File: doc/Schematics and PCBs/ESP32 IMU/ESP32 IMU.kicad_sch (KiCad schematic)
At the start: 7 parts, among them J1 +5V, U1 BA50JC5T

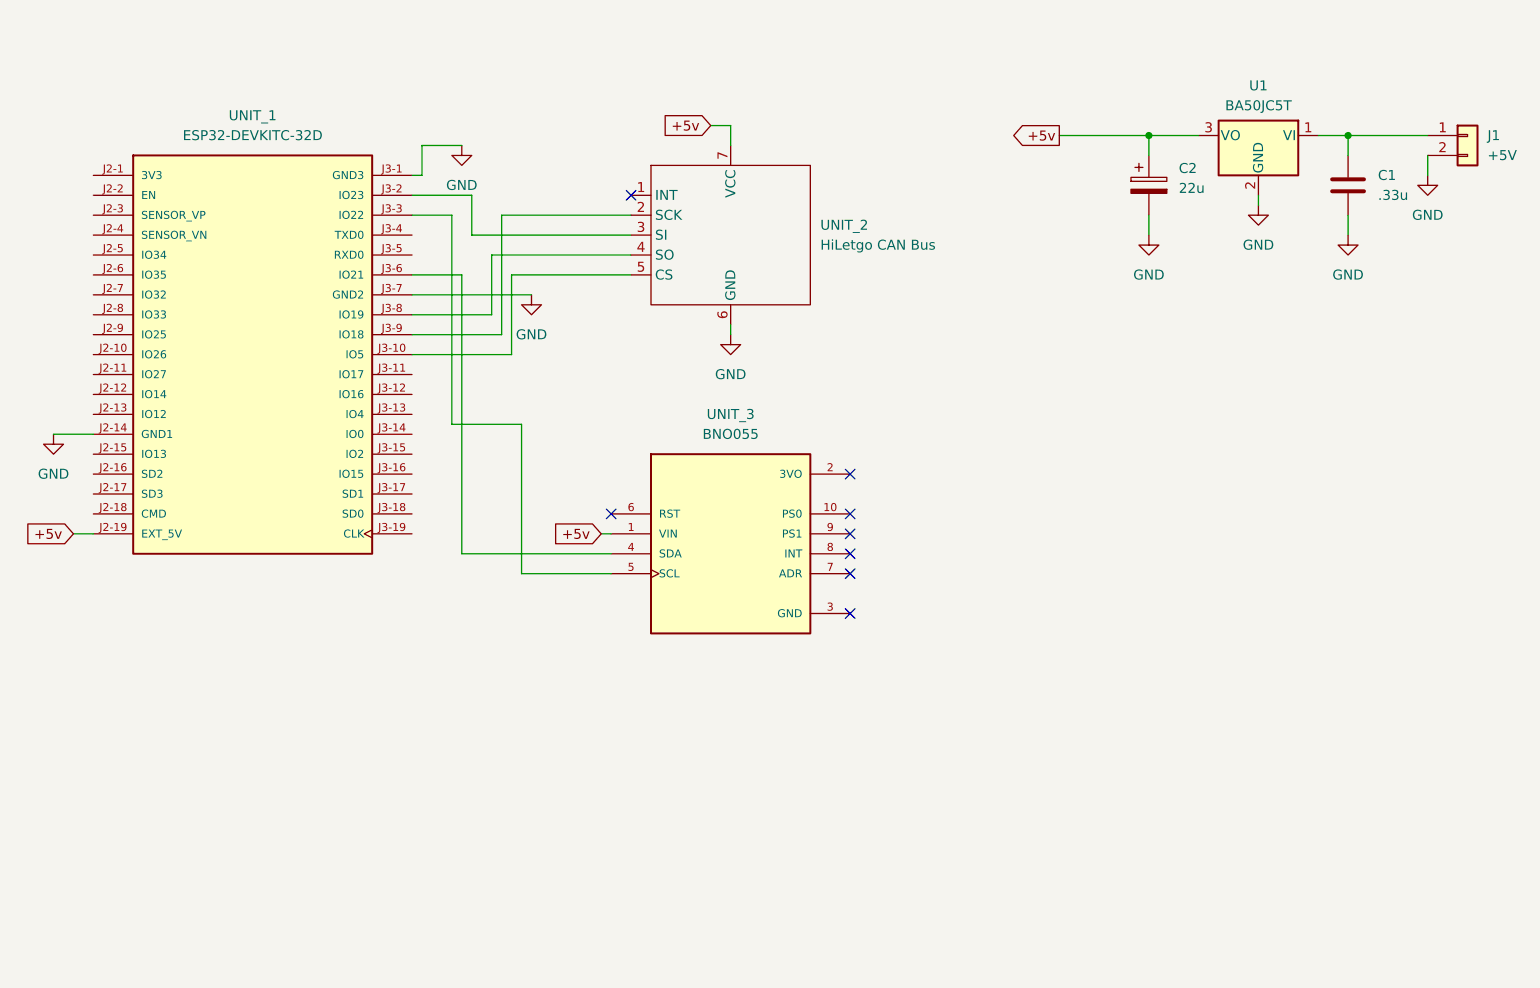
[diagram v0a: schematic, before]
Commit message: Final Touches on IMU
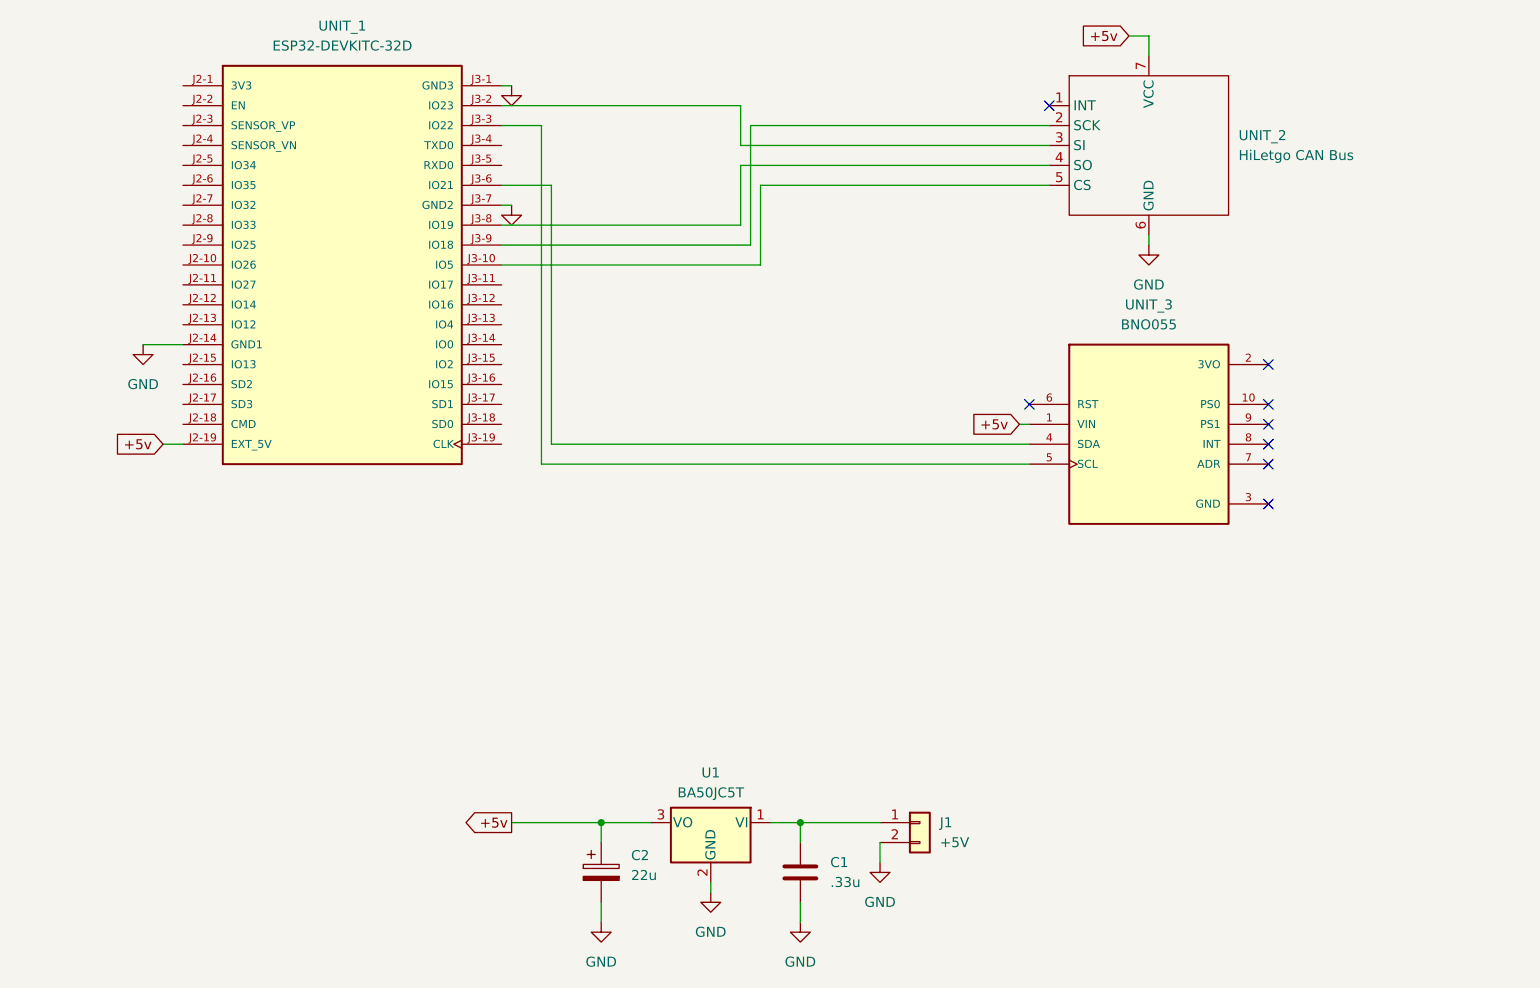
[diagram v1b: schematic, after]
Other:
- moved on the sheet: C1, C2, J1, U1, UNIT_1, UNIT_2, UNIT_3
